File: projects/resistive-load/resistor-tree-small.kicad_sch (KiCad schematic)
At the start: 27 parts, among them Q35 SSM3K333R, Q36 SSM3K333R, Q37 SSM3K333R, Q38 SSM3K333R, Q39 SSM3K333R

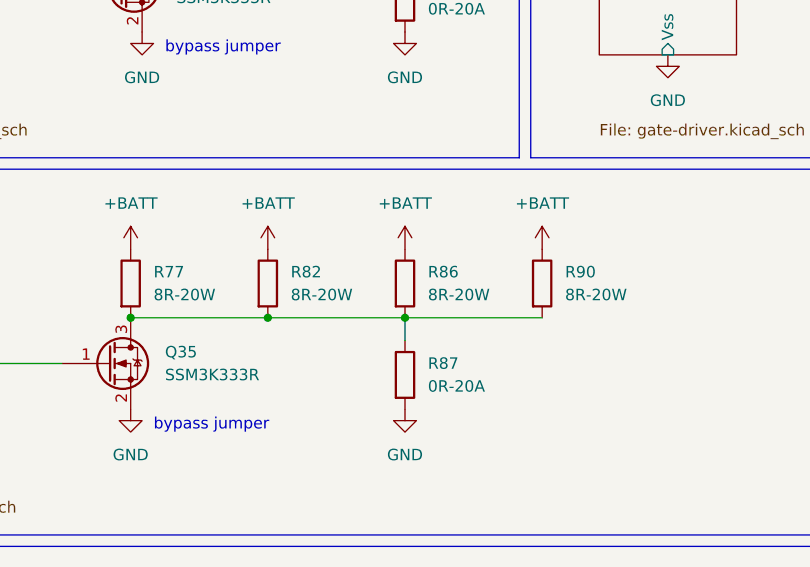
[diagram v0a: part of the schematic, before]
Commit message: Ayo
Ayo
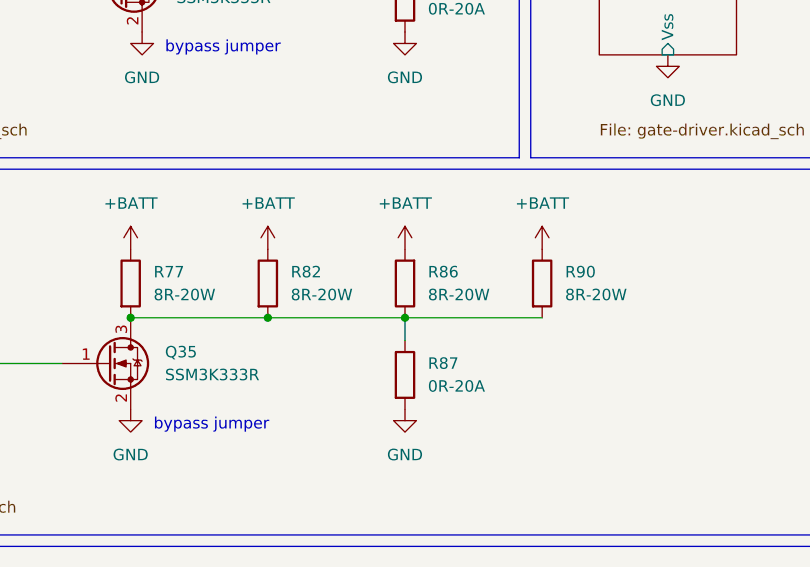
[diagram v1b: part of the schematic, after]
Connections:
- net +BATT: now also R86.2; no longer R86.1
- net at Q35.3 (D), R77.2, R82.2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: now also R86.1; no longer R86.2
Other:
- moved on the sheet: R86
